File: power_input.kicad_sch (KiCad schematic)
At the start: 17 parts, among them J1 PWR_24V_IN, J2 PWR_12V_IN, J3 PWR_5V_IN, J4 PWR_±15V_IN

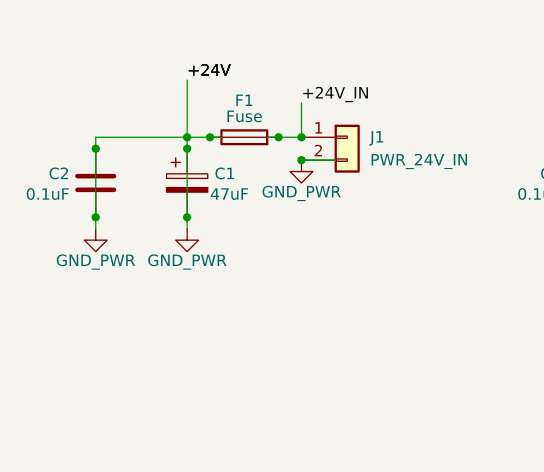
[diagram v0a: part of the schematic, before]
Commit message: im so happy
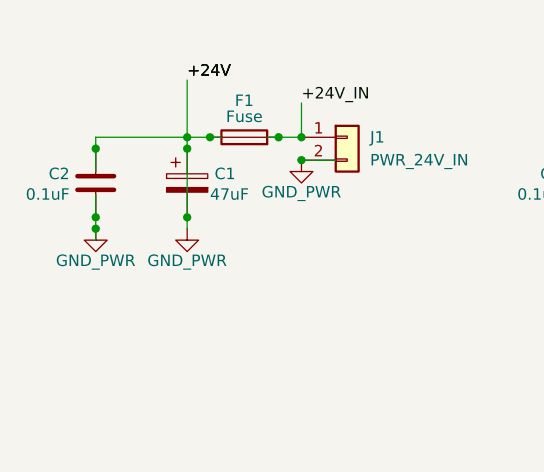
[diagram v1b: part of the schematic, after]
